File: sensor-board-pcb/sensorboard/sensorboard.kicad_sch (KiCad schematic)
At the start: 19 parts, among them J1 TO_MOTHERBOARD, J10 PZT_08, J11 PZT_09, J12 PZT_10, J13 PZT_11, J14 PZT_12, J15 PZT_13, J16 PZT_14, J17 PZT_15, J2 PZT_00, J3 PZT_01, J4 PZT_02, J5 PZT_03, J6 PZT_04, J7 PZT_05, J8 PZT_06, J9 PZT_07, U1 CD74HC4067M

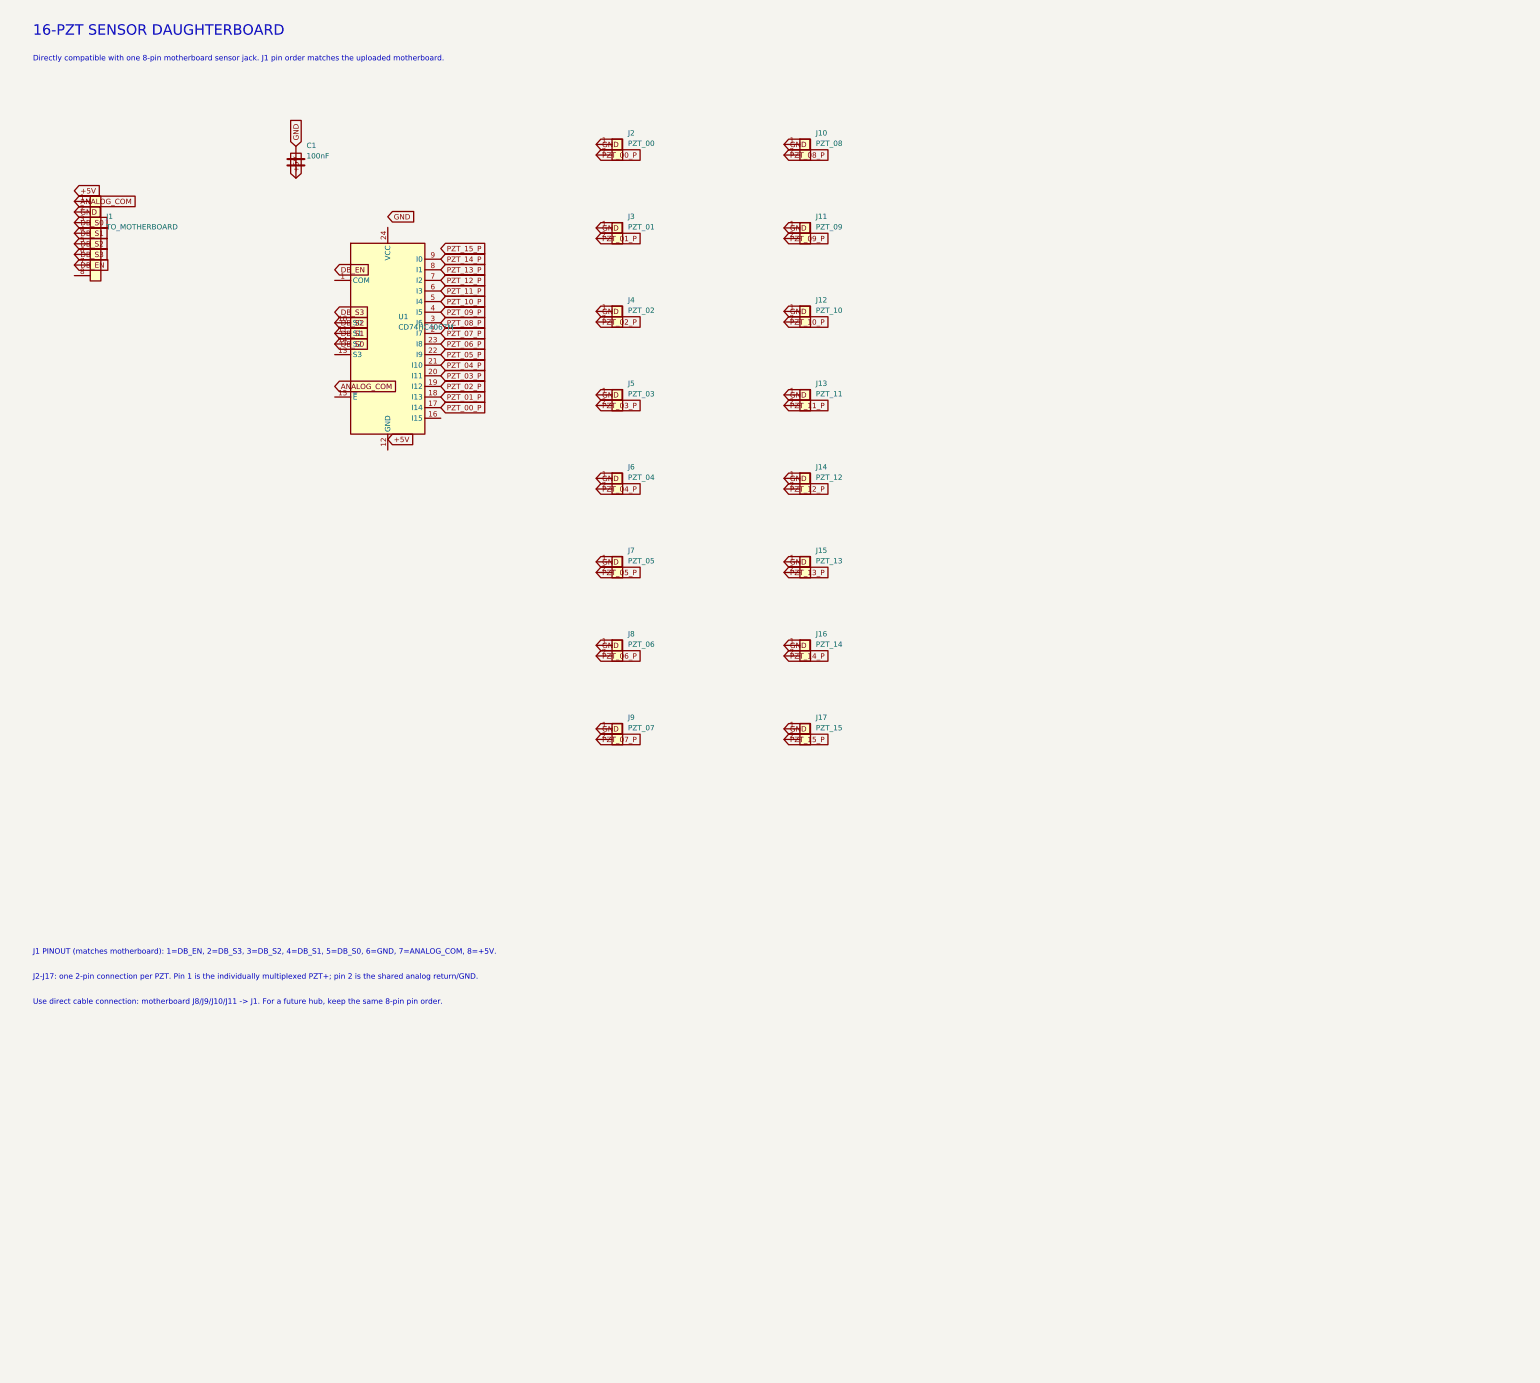
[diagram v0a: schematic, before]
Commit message: routing fixed
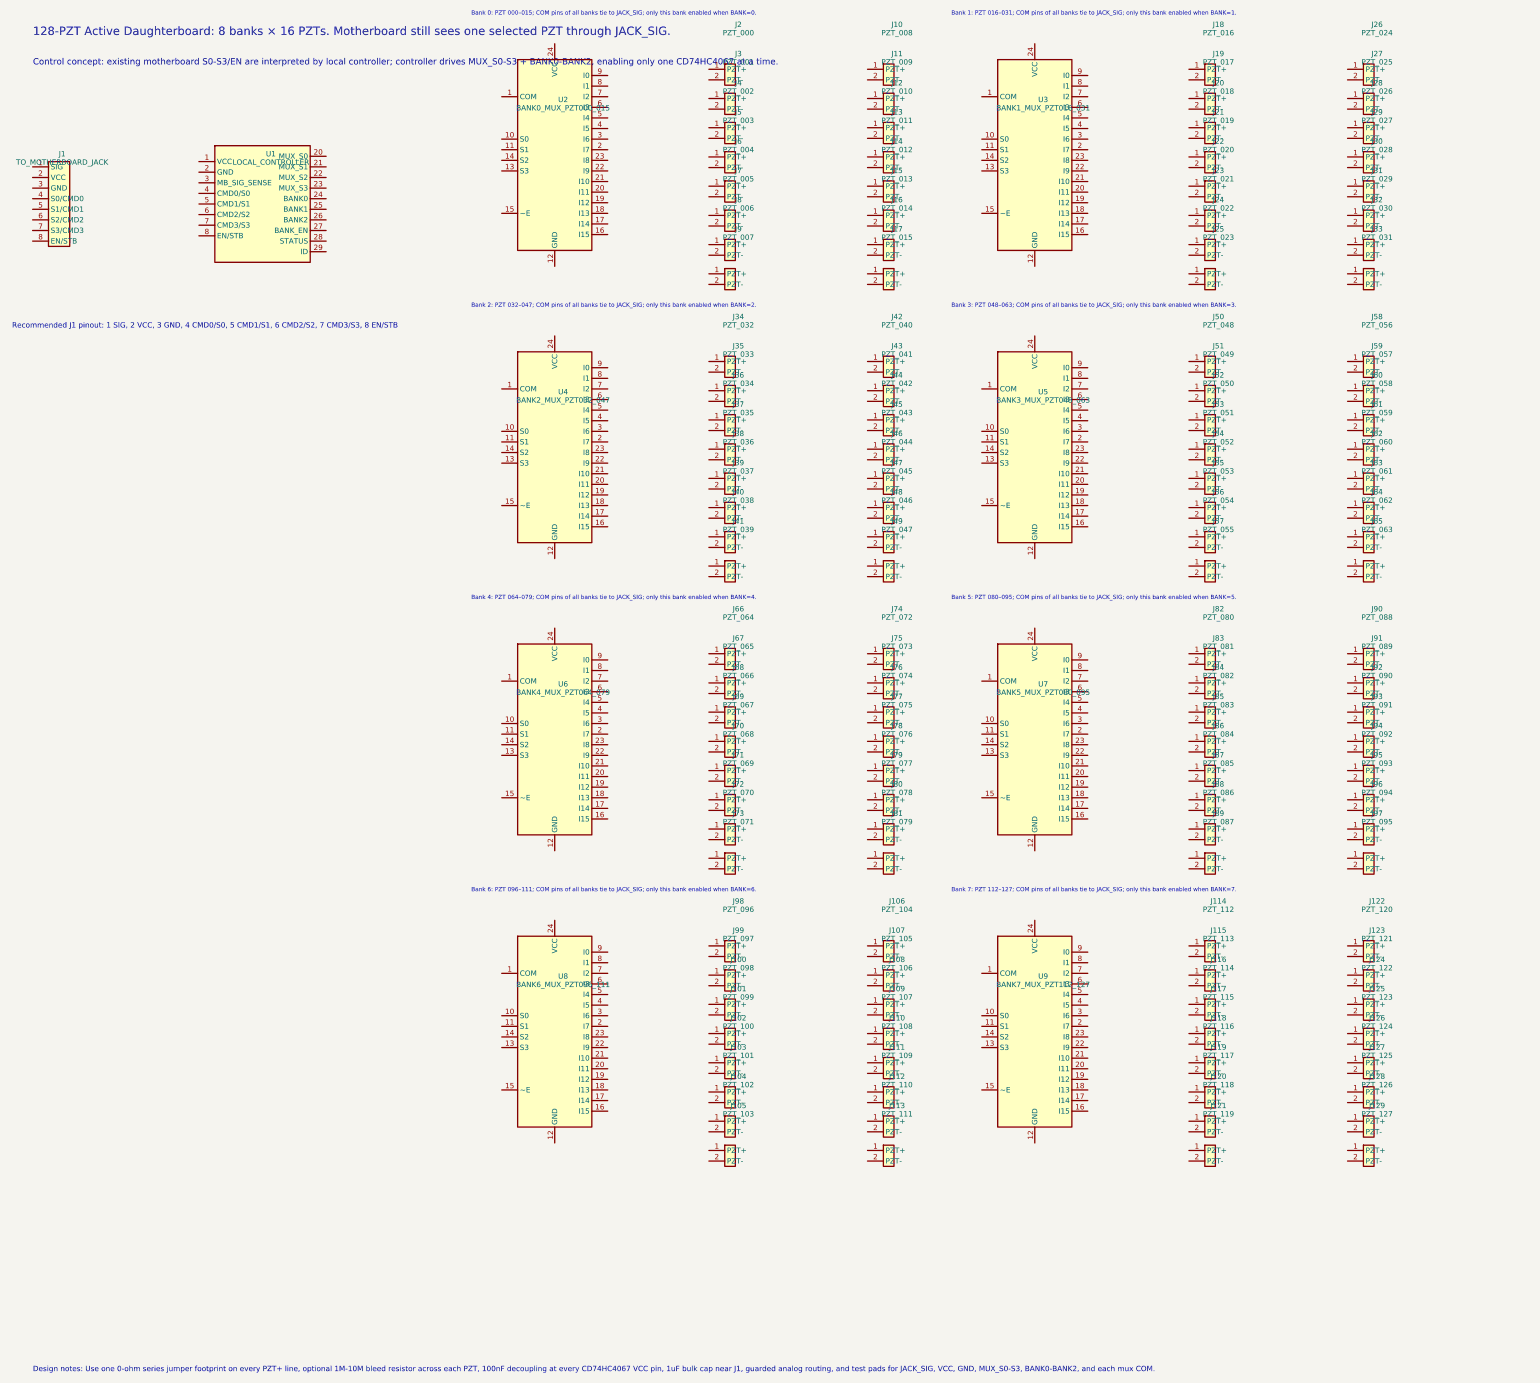
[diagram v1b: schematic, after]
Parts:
- removed C1: 100nF, Capacitor_SMD:C_0603_1608Metric, symbol Device:C
- removed J1: TO_MOTHERBOARD, Connector_Molex:Molex_Micro-Fit_3.0_43650-0815_1x08_P3.00mm_Vertical, symbol Connector_Generic:Conn_01x08
- removed J10: PZT_08, Connector_PinHeader_2.54mm:PinHeader_1x02_P2.54mm_Vertical, symbol Connector_Generic:Conn_01x02
- removed J11: PZT_09, Connector_PinHeader_2.54mm:PinHeader_1x02_P2.54mm_Vertical, symbol Connector_Generic:Conn_01x02
- removed J12: PZT_10, Connector_PinHeader_2.54mm:PinHeader_1x02_P2.54mm_Vertical, symbol Connector_Generic:Conn_01x02
- removed J13: PZT_11, Connector_PinHeader_2.54mm:PinHeader_1x02_P2.54mm_Vertical, symbol Connector_Generic:Conn_01x02
- removed J14: PZT_12, Connector_PinHeader_2.54mm:PinHeader_1x02_P2.54mm_Vertical, symbol Connector_Generic:Conn_01x02
- removed J15: PZT_13, Connector_PinHeader_2.54mm:PinHeader_1x02_P2.54mm_Vertical, symbol Connector_Generic:Conn_01x02
- removed J16: PZT_14, Connector_PinHeader_2.54mm:PinHeader_1x02_P2.54mm_Vertical, symbol Connector_Generic:Conn_01x02
- removed J17: PZT_15, Connector_PinHeader_2.54mm:PinHeader_1x02_P2.54mm_Vertical, symbol Connector_Generic:Conn_01x02
- removed J2: PZT_00, Connector_PinHeader_2.54mm:PinHeader_1x02_P2.54mm_Vertical, symbol Connector_Generic:Conn_01x02
- removed J3: PZT_01, Connector_PinHeader_2.54mm:PinHeader_1x02_P2.54mm_Vertical, symbol Connector_Generic:Conn_01x02
- removed J4: PZT_02, Connector_PinHeader_2.54mm:PinHeader_1x02_P2.54mm_Vertical, symbol Connector_Generic:Conn_01x02
- removed J5: PZT_03, Connector_PinHeader_2.54mm:PinHeader_1x02_P2.54mm_Vertical, symbol Connector_Generic:Conn_01x02
- removed J6: PZT_04, Connector_PinHeader_2.54mm:PinHeader_1x02_P2.54mm_Vertical, symbol Connector_Generic:Conn_01x02
- removed J7: PZT_05, Connector_PinHeader_2.54mm:PinHeader_1x02_P2.54mm_Vertical, symbol Connector_Generic:Conn_01x02
- removed J8: PZT_06, Connector_PinHeader_2.54mm:PinHeader_1x02_P2.54mm_Vertical, symbol Connector_Generic:Conn_01x02
- removed J9: PZT_07, Connector_PinHeader_2.54mm:PinHeader_1x02_P2.54mm_Vertical, symbol Connector_Generic:Conn_01x02
- removed U1: CD74HC4067M, Package_SO:SOIC-24W_7.5x15.4mm_P1.27mm, symbol 74xx:CD74HC4067M
- added J1: TO_MOTHERBOARD_JACK, Connector_PinHeader_2.54mm:PinHeader_1x08_P2.54mm_Vertical, symbol Daughter:MicroFit_01x08_Motherboard
- added J10: PZT_008, Connector_PinHeader_2.54mm:PinHeader_1x02_P2.54mm_Vertical, symbol Daughter:PZT_Conn_01x02
- added J100: PZT_098, Connector_PinHeader_2.54mm:PinHeader_1x02_P2.54mm_Vertical, symbol Daughter:PZT_Conn_01x02
- added J101: PZT_099, Connector_PinHeader_2.54mm:PinHeader_1x02_P2.54mm_Vertical, symbol Daughter:PZT_Conn_01x02
- added J102: PZT_100, Connector_PinHeader_2.54mm:PinHeader_1x02_P2.54mm_Vertical, symbol Daughter:PZT_Conn_01x02
- added J103: PZT_101, Connector_PinHeader_2.54mm:PinHeader_1x02_P2.54mm_Vertical, symbol Daughter:PZT_Conn_01x02
- added J104: PZT_102, Connector_PinHeader_2.54mm:PinHeader_1x02_P2.54mm_Vertical, symbol Daughter:PZT_Conn_01x02
- added J105: PZT_103, Connector_PinHeader_2.54mm:PinHeader_1x02_P2.54mm_Vertical, symbol Daughter:PZT_Conn_01x02
- added J106: PZT_104, Connector_PinHeader_2.54mm:PinHeader_1x02_P2.54mm_Vertical, symbol Daughter:PZT_Conn_01x02
- added J107: PZT_105, Connector_PinHeader_2.54mm:PinHeader_1x02_P2.54mm_Vertical, symbol Daughter:PZT_Conn_01x02
- added J108: PZT_106, Connector_PinHeader_2.54mm:PinHeader_1x02_P2.54mm_Vertical, symbol Daughter:PZT_Conn_01x02
- added J109: PZT_107, Connector_PinHeader_2.54mm:PinHeader_1x02_P2.54mm_Vertical, symbol Daughter:PZT_Conn_01x02
- added J11: PZT_009, Connector_PinHeader_2.54mm:PinHeader_1x02_P2.54mm_Vertical, symbol Daughter:PZT_Conn_01x02
- added J110: PZT_108, Connector_PinHeader_2.54mm:PinHeader_1x02_P2.54mm_Vertical, symbol Daughter:PZT_Conn_01x02
- added J111: PZT_109, Connector_PinHeader_2.54mm:PinHeader_1x02_P2.54mm_Vertical, symbol Daughter:PZT_Conn_01x02
- added J112: PZT_110, Connector_PinHeader_2.54mm:PinHeader_1x02_P2.54mm_Vertical, symbol Daughter:PZT_Conn_01x02
- added J113: PZT_111, Connector_PinHeader_2.54mm:PinHeader_1x02_P2.54mm_Vertical, symbol Daughter:PZT_Conn_01x02
- added J114: PZT_112, Connector_PinHeader_2.54mm:PinHeader_1x02_P2.54mm_Vertical, symbol Daughter:PZT_Conn_01x02
- added J115: PZT_113, Connector_PinHeader_2.54mm:PinHeader_1x02_P2.54mm_Vertical, symbol Daughter:PZT_Conn_01x02
- added J116: PZT_114, Connector_PinHeader_2.54mm:PinHeader_1x02_P2.54mm_Vertical, symbol Daughter:PZT_Conn_01x02
- added J117: PZT_115, Connector_PinHeader_2.54mm:PinHeader_1x02_P2.54mm_Vertical, symbol Daughter:PZT_Conn_01x02
- added J118: PZT_116, Connector_PinHeader_2.54mm:PinHeader_1x02_P2.54mm_Vertical, symbol Daughter:PZT_Conn_01x02
- added J119: PZT_117, Connector_PinHeader_2.54mm:PinHeader_1x02_P2.54mm_Vertical, symbol Daughter:PZT_Conn_01x02
- added J12: PZT_010, Connector_PinHeader_2.54mm:PinHeader_1x02_P2.54mm_Vertical, symbol Daughter:PZT_Conn_01x02
- added J120: PZT_118, Connector_PinHeader_2.54mm:PinHeader_1x02_P2.54mm_Vertical, symbol Daughter:PZT_Conn_01x02
- added J121: PZT_119, Connector_PinHeader_2.54mm:PinHeader_1x02_P2.54mm_Vertical, symbol Daughter:PZT_Conn_01x02
- added J122: PZT_120, Connector_PinHeader_2.54mm:PinHeader_1x02_P2.54mm_Vertical, symbol Daughter:PZT_Conn_01x02
- added J123: PZT_121, Connector_PinHeader_2.54mm:PinHeader_1x02_P2.54mm_Vertical, symbol Daughter:PZT_Conn_01x02
- added J124: PZT_122, Connector_PinHeader_2.54mm:PinHeader_1x02_P2.54mm_Vertical, symbol Daughter:PZT_Conn_01x02
- added J125: PZT_123, Connector_PinHeader_2.54mm:PinHeader_1x02_P2.54mm_Vertical, symbol Daughter:PZT_Conn_01x02
- added J126: PZT_124, Connector_PinHeader_2.54mm:PinHeader_1x02_P2.54mm_Vertical, symbol Daughter:PZT_Conn_01x02
- added J127: PZT_125, Connector_PinHeader_2.54mm:PinHeader_1x02_P2.54mm_Vertical, symbol Daughter:PZT_Conn_01x02
- added J128: PZT_126, Connector_PinHeader_2.54mm:PinHeader_1x02_P2.54mm_Vertical, symbol Daughter:PZT_Conn_01x02
- added J129: PZT_127, Connector_PinHeader_2.54mm:PinHeader_1x02_P2.54mm_Vertical, symbol Daughter:PZT_Conn_01x02
- added J13: PZT_011, Connector_PinHeader_2.54mm:PinHeader_1x02_P2.54mm_Vertical, symbol Daughter:PZT_Conn_01x02
- added J14: PZT_012, Connector_PinHeader_2.54mm:PinHeader_1x02_P2.54mm_Vertical, symbol Daughter:PZT_Conn_01x02
- added J15: PZT_013, Connector_PinHeader_2.54mm:PinHeader_1x02_P2.54mm_Vertical, symbol Daughter:PZT_Conn_01x02
- added J16: PZT_014, Connector_PinHeader_2.54mm:PinHeader_1x02_P2.54mm_Vertical, symbol Daughter:PZT_Conn_01x02
- added J17: PZT_015, Connector_PinHeader_2.54mm:PinHeader_1x02_P2.54mm_Vertical, symbol Daughter:PZT_Conn_01x02
- added J18: PZT_016, Connector_PinHeader_2.54mm:PinHeader_1x02_P2.54mm_Vertical, symbol Daughter:PZT_Conn_01x02
- added J19: PZT_017, Connector_PinHeader_2.54mm:PinHeader_1x02_P2.54mm_Vertical, symbol Daughter:PZT_Conn_01x02
- added J2: PZT_000, Connector_PinHeader_2.54mm:PinHeader_1x02_P2.54mm_Vertical, symbol Daughter:PZT_Conn_01x02
- added J20: PZT_018, Connector_PinHeader_2.54mm:PinHeader_1x02_P2.54mm_Vertical, symbol Daughter:PZT_Conn_01x02
- added J21: PZT_019, Connector_PinHeader_2.54mm:PinHeader_1x02_P2.54mm_Vertical, symbol Daughter:PZT_Conn_01x02
- added J22: PZT_020, Connector_PinHeader_2.54mm:PinHeader_1x02_P2.54mm_Vertical, symbol Daughter:PZT_Conn_01x02
- added J23: PZT_021, Connector_PinHeader_2.54mm:PinHeader_1x02_P2.54mm_Vertical, symbol Daughter:PZT_Conn_01x02
- added J24: PZT_022, Connector_PinHeader_2.54mm:PinHeader_1x02_P2.54mm_Vertical, symbol Daughter:PZT_Conn_01x02
- added J25: PZT_023, Connector_PinHeader_2.54mm:PinHeader_1x02_P2.54mm_Vertical, symbol Daughter:PZT_Conn_01x02
- added J26: PZT_024, Connector_PinHeader_2.54mm:PinHeader_1x02_P2.54mm_Vertical, symbol Daughter:PZT_Conn_01x02
- added J27: PZT_025, Connector_PinHeader_2.54mm:PinHeader_1x02_P2.54mm_Vertical, symbol Daughter:PZT_Conn_01x02
- added J28: PZT_026, Connector_PinHeader_2.54mm:PinHeader_1x02_P2.54mm_Vertical, symbol Daughter:PZT_Conn_01x02
- added J29: PZT_027, Connector_PinHeader_2.54mm:PinHeader_1x02_P2.54mm_Vertical, symbol Daughter:PZT_Conn_01x02
- added J3: PZT_001, Connector_PinHeader_2.54mm:PinHeader_1x02_P2.54mm_Vertical, symbol Daughter:PZT_Conn_01x02
- added J30: PZT_028, Connector_PinHeader_2.54mm:PinHeader_1x02_P2.54mm_Vertical, symbol Daughter:PZT_Conn_01x02
- added J31: PZT_029, Connector_PinHeader_2.54mm:PinHeader_1x02_P2.54mm_Vertical, symbol Daughter:PZT_Conn_01x02
- added J32: PZT_030, Connector_PinHeader_2.54mm:PinHeader_1x02_P2.54mm_Vertical, symbol Daughter:PZT_Conn_01x02
- added J33: PZT_031, Connector_PinHeader_2.54mm:PinHeader_1x02_P2.54mm_Vertical, symbol Daughter:PZT_Conn_01x02
- added J34: PZT_032, Connector_PinHeader_2.54mm:PinHeader_1x02_P2.54mm_Vertical, symbol Daughter:PZT_Conn_01x02
- added J35: PZT_033, Connector_PinHeader_2.54mm:PinHeader_1x02_P2.54mm_Vertical, symbol Daughter:PZT_Conn_01x02
- added J36: PZT_034, Connector_PinHeader_2.54mm:PinHeader_1x02_P2.54mm_Vertical, symbol Daughter:PZT_Conn_01x02
- added J37: PZT_035, Connector_PinHeader_2.54mm:PinHeader_1x02_P2.54mm_Vertical, symbol Daughter:PZT_Conn_01x02
- added J38: PZT_036, Connector_PinHeader_2.54mm:PinHeader_1x02_P2.54mm_Vertical, symbol Daughter:PZT_Conn_01x02
- added J39: PZT_037, Connector_PinHeader_2.54mm:PinHeader_1x02_P2.54mm_Vertical, symbol Daughter:PZT_Conn_01x02
- added J4: PZT_002, Connector_PinHeader_2.54mm:PinHeader_1x02_P2.54mm_Vertical, symbol Daughter:PZT_Conn_01x02
- added J40: PZT_038, Connector_PinHeader_2.54mm:PinHeader_1x02_P2.54mm_Vertical, symbol Daughter:PZT_Conn_01x02
- added J41: PZT_039, Connector_PinHeader_2.54mm:PinHeader_1x02_P2.54mm_Vertical, symbol Daughter:PZT_Conn_01x02
- added J42: PZT_040, Connector_PinHeader_2.54mm:PinHeader_1x02_P2.54mm_Vertical, symbol Daughter:PZT_Conn_01x02
- added J43: PZT_041, Connector_PinHeader_2.54mm:PinHeader_1x02_P2.54mm_Vertical, symbol Daughter:PZT_Conn_01x02
- added J44: PZT_042, Connector_PinHeader_2.54mm:PinHeader_1x02_P2.54mm_Vertical, symbol Daughter:PZT_Conn_01x02
- added J45: PZT_043, Connector_PinHeader_2.54mm:PinHeader_1x02_P2.54mm_Vertical, symbol Daughter:PZT_Conn_01x02
- added J46: PZT_044, Connector_PinHeader_2.54mm:PinHeader_1x02_P2.54mm_Vertical, symbol Daughter:PZT_Conn_01x02
- added J47: PZT_045, Connector_PinHeader_2.54mm:PinHeader_1x02_P2.54mm_Vertical, symbol Daughter:PZT_Conn_01x02
- added J48: PZT_046, Connector_PinHeader_2.54mm:PinHeader_1x02_P2.54mm_Vertical, symbol Daughter:PZT_Conn_01x02
- added J49: PZT_047, Connector_PinHeader_2.54mm:PinHeader_1x02_P2.54mm_Vertical, symbol Daughter:PZT_Conn_01x02
- added J5: PZT_003, Connector_PinHeader_2.54mm:PinHeader_1x02_P2.54mm_Vertical, symbol Daughter:PZT_Conn_01x02
- added J50: PZT_048, Connector_PinHeader_2.54mm:PinHeader_1x02_P2.54mm_Vertical, symbol Daughter:PZT_Conn_01x02
- added J51: PZT_049, Connector_PinHeader_2.54mm:PinHeader_1x02_P2.54mm_Vertical, symbol Daughter:PZT_Conn_01x02
- added J52: PZT_050, Connector_PinHeader_2.54mm:PinHeader_1x02_P2.54mm_Vertical, symbol Daughter:PZT_Conn_01x02
- added J53: PZT_051, Connector_PinHeader_2.54mm:PinHeader_1x02_P2.54mm_Vertical, symbol Daughter:PZT_Conn_01x02
- added J54: PZT_052, Connector_PinHeader_2.54mm:PinHeader_1x02_P2.54mm_Vertical, symbol Daughter:PZT_Conn_01x02
- added J55: PZT_053, Connector_PinHeader_2.54mm:PinHeader_1x02_P2.54mm_Vertical, symbol Daughter:PZT_Conn_01x02
- added J56: PZT_054, Connector_PinHeader_2.54mm:PinHeader_1x02_P2.54mm_Vertical, symbol Daughter:PZT_Conn_01x02
- added J57: PZT_055, Connector_PinHeader_2.54mm:PinHeader_1x02_P2.54mm_Vertical, symbol Daughter:PZT_Conn_01x02
- added J58: PZT_056, Connector_PinHeader_2.54mm:PinHeader_1x02_P2.54mm_Vertical, symbol Daughter:PZT_Conn_01x02
- added J59: PZT_057, Connector_PinHeader_2.54mm:PinHeader_1x02_P2.54mm_Vertical, symbol Daughter:PZT_Conn_01x02
- added J6: PZT_004, Connector_PinHeader_2.54mm:PinHeader_1x02_P2.54mm_Vertical, symbol Daughter:PZT_Conn_01x02
- added J60: PZT_058, Connector_PinHeader_2.54mm:PinHeader_1x02_P2.54mm_Vertical, symbol Daughter:PZT_Conn_01x02
- added J61: PZT_059, Connector_PinHeader_2.54mm:PinHeader_1x02_P2.54mm_Vertical, symbol Daughter:PZT_Conn_01x02
- added J62: PZT_060, Connector_PinHeader_2.54mm:PinHeader_1x02_P2.54mm_Vertical, symbol Daughter:PZT_Conn_01x02
- added J63: PZT_061, Connector_PinHeader_2.54mm:PinHeader_1x02_P2.54mm_Vertical, symbol Daughter:PZT_Conn_01x02
- added J64: PZT_062, Connector_PinHeader_2.54mm:PinHeader_1x02_P2.54mm_Vertical, symbol Daughter:PZT_Conn_01x02
- added J65: PZT_063, Connector_PinHeader_2.54mm:PinHeader_1x02_P2.54mm_Vertical, symbol Daughter:PZT_Conn_01x02
- added J66: PZT_064, Connector_PinHeader_2.54mm:PinHeader_1x02_P2.54mm_Vertical, symbol Daughter:PZT_Conn_01x02
- added J67: PZT_065, Connector_PinHeader_2.54mm:PinHeader_1x02_P2.54mm_Vertical, symbol Daughter:PZT_Conn_01x02
- added J68: PZT_066, Connector_PinHeader_2.54mm:PinHeader_1x02_P2.54mm_Vertical, symbol Daughter:PZT_Conn_01x02
- added J69: PZT_067, Connector_PinHeader_2.54mm:PinHeader_1x02_P2.54mm_Vertical, symbol Daughter:PZT_Conn_01x02
- added J7: PZT_005, Connector_PinHeader_2.54mm:PinHeader_1x02_P2.54mm_Vertical, symbol Daughter:PZT_Conn_01x02
- added J70: PZT_068, Connector_PinHeader_2.54mm:PinHeader_1x02_P2.54mm_Vertical, symbol Daughter:PZT_Conn_01x02
- added J71: PZT_069, Connector_PinHeader_2.54mm:PinHeader_1x02_P2.54mm_Vertical, symbol Daughter:PZT_Conn_01x02
- added J72: PZT_070, Connector_PinHeader_2.54mm:PinHeader_1x02_P2.54mm_Vertical, symbol Daughter:PZT_Conn_01x02
- added J73: PZT_071, Connector_PinHeader_2.54mm:PinHeader_1x02_P2.54mm_Vertical, symbol Daughter:PZT_Conn_01x02
- added J74: PZT_072, Connector_PinHeader_2.54mm:PinHeader_1x02_P2.54mm_Vertical, symbol Daughter:PZT_Conn_01x02
- added J75: PZT_073, Connector_PinHeader_2.54mm:PinHeader_1x02_P2.54mm_Vertical, symbol Daughter:PZT_Conn_01x02
- added J76: PZT_074, Connector_PinHeader_2.54mm:PinHeader_1x02_P2.54mm_Vertical, symbol Daughter:PZT_Conn_01x02
- added J77: PZT_075, Connector_PinHeader_2.54mm:PinHeader_1x02_P2.54mm_Vertical, symbol Daughter:PZT_Conn_01x02
- added J78: PZT_076, Connector_PinHeader_2.54mm:PinHeader_1x02_P2.54mm_Vertical, symbol Daughter:PZT_Conn_01x02
- added J79: PZT_077, Connector_PinHeader_2.54mm:PinHeader_1x02_P2.54mm_Vertical, symbol Daughter:PZT_Conn_01x02
- added J8: PZT_006, Connector_PinHeader_2.54mm:PinHeader_1x02_P2.54mm_Vertical, symbol Daughter:PZT_Conn_01x02
- added J80: PZT_078, Connector_PinHeader_2.54mm:PinHeader_1x02_P2.54mm_Vertical, symbol Daughter:PZT_Conn_01x02
- added J81: PZT_079, Connector_PinHeader_2.54mm:PinHeader_1x02_P2.54mm_Vertical, symbol Daughter:PZT_Conn_01x02
- added J82: PZT_080, Connector_PinHeader_2.54mm:PinHeader_1x02_P2.54mm_Vertical, symbol Daughter:PZT_Conn_01x02
- added J83: PZT_081, Connector_PinHeader_2.54mm:PinHeader_1x02_P2.54mm_Vertical, symbol Daughter:PZT_Conn_01x02
- added J84: PZT_082, Connector_PinHeader_2.54mm:PinHeader_1x02_P2.54mm_Vertical, symbol Daughter:PZT_Conn_01x02
- added J85: PZT_083, Connector_PinHeader_2.54mm:PinHeader_1x02_P2.54mm_Vertical, symbol Daughter:PZT_Conn_01x02
- added J86: PZT_084, Connector_PinHeader_2.54mm:PinHeader_1x02_P2.54mm_Vertical, symbol Daughter:PZT_Conn_01x02
- added J87: PZT_085, Connector_PinHeader_2.54mm:PinHeader_1x02_P2.54mm_Vertical, symbol Daughter:PZT_Conn_01x02
- added J88: PZT_086, Connector_PinHeader_2.54mm:PinHeader_1x02_P2.54mm_Vertical, symbol Daughter:PZT_Conn_01x02
- added J89: PZT_087, Connector_PinHeader_2.54mm:PinHeader_1x02_P2.54mm_Vertical, symbol Daughter:PZT_Conn_01x02
- added J9: PZT_007, Connector_PinHeader_2.54mm:PinHeader_1x02_P2.54mm_Vertical, symbol Daughter:PZT_Conn_01x02
- added J90: PZT_088, Connector_PinHeader_2.54mm:PinHeader_1x02_P2.54mm_Vertical, symbol Daughter:PZT_Conn_01x02
- added J91: PZT_089, Connector_PinHeader_2.54mm:PinHeader_1x02_P2.54mm_Vertical, symbol Daughter:PZT_Conn_01x02
- added J92: PZT_090, Connector_PinHeader_2.54mm:PinHeader_1x02_P2.54mm_Vertical, symbol Daughter:PZT_Conn_01x02
- added J93: PZT_091, Connector_PinHeader_2.54mm:PinHeader_1x02_P2.54mm_Vertical, symbol Daughter:PZT_Conn_01x02
- added J94: PZT_092, Connector_PinHeader_2.54mm:PinHeader_1x02_P2.54mm_Vertical, symbol Daughter:PZT_Conn_01x02
- added J95: PZT_093, Connector_PinHeader_2.54mm:PinHeader_1x02_P2.54mm_Vertical, symbol Daughter:PZT_Conn_01x02
- added J96: PZT_094, Connector_PinHeader_2.54mm:PinHeader_1x02_P2.54mm_Vertical, symbol Daughter:PZT_Conn_01x02
- added J97: PZT_095, Connector_PinHeader_2.54mm:PinHeader_1x02_P2.54mm_Vertical, symbol Daughter:PZT_Conn_01x02
- added J98: PZT_096, Connector_PinHeader_2.54mm:PinHeader_1x02_P2.54mm_Vertical, symbol Daughter:PZT_Conn_01x02
- added J99: PZT_097, Connector_PinHeader_2.54mm:PinHeader_1x02_P2.54mm_Vertical, symbol Daughter:PZT_Conn_01x02
- added U1: LOCAL_CONTROLLER, Package_DIP:DIP-20_W7.62mm, symbol Daughter:Local_Controller_or_GPIO
- added U2: BANK0_MUX_PZT000_015, Package_SO:SOIC-24W_7.5x15.4mm_P1.27mm, symbol Daughter:CD74HC4067M
- added U3: BANK1_MUX_PZT016_031, Package_SO:SOIC-24W_7.5x15.4mm_P1.27mm, symbol Daughter:CD74HC4067M
- added U4: BANK2_MUX_PZT032_047, Package_SO:SOIC-24W_7.5x15.4mm_P1.27mm, symbol Daughter:CD74HC4067M
- added U5: BANK3_MUX_PZT048_063, Package_SO:SOIC-24W_7.5x15.4mm_P1.27mm, symbol Daughter:CD74HC4067M
- added U6: BANK4_MUX_PZT064_079, Package_SO:SOIC-24W_7.5x15.4mm_P1.27mm, symbol Daughter:CD74HC4067M
- added U7: BANK5_MUX_PZT080_095, Package_SO:SOIC-24W_7.5x15.4mm_P1.27mm, symbol Daughter:CD74HC4067M
- added U8: BANK6_MUX_PZT096_111, Package_SO:SOIC-24W_7.5x15.4mm_P1.27mm, symbol Daughter:CD74HC4067M
- added U9: BANK7_MUX_PZT112_127, Package_SO:SOIC-24W_7.5x15.4mm_P1.27mm, symbol Daughter:CD74HC4067M
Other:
- note added: "128-PZT Active Daughterboard: 8 banks × 16 PZTs. Motherboard still sees one selected PZT through JACK_SIG."
- note added: "Bank 0: PZT 000–015; COM pins of all banks tie to JACK_SIG; only this bank enabled when BANK=0."
- note added: "Bank 1: PZT 016–031; COM pins of all banks tie to JACK_SIG; only this bank enabled when BANK=1."
- note added: "Bank 2: PZT 032–047; COM pins of all banks tie to JACK_SIG; only this bank enabled when BANK=2."
- note added: "Bank 3: PZT 048–063; COM pins of all banks tie to JACK_SIG; only this bank enabled when BANK=3."
- note added: "Bank 4: PZT 064–079; COM pins of all banks tie to JACK_SIG; only this bank enabled when BANK=4."
- note added: "Bank 5: PZT 080–095; COM pins of all banks tie to JACK_SIG; only this bank enabled when BANK=5."
- note added: "Bank 6: PZT 096–111; COM pins of all banks tie to JACK_SIG; only this bank enabled when BANK=6."
- note added: "Bank 7: PZT 112–127; COM pins of all banks tie to JACK_SIG; only this bank enabled when BANK=7."
- note added: "Control concept: existing motherboard S0-S3/EN are interpreted by local controller; controller drives MUX_S0-S3 + BANK0-BANK2, enabling only one CD74HC4067 at a time."
- note added: "Design notes: Use one 0-ohm series jumper footprint on every PZT+ line, optional 1M-10M bleed resistor across each PZT, 100nF decoupling at every CD74HC4067 VCC pin, 1uF bulk cap near J1, guarded analog routing, and test pads for JACK_SIG, VCC, GND, MUX_S0-S3, BANK0-BANK2, and each mux COM."
- note added: "Recommended J1 pinout: 1 SIG, 2 VCC, 3 GND, 4 CMD0/S0, 5 CMD1/S1, 6 CMD2/S2, 7 CMD3/S3, 8 EN/STB"
- note removed: "16-PZT SENSOR DAUGHTERBOARD"
- note removed: "Directly compatible with one 8-pin motherboard sensor jack. J1 pin order matches the uploaded motherboard."
- note removed: "J1 PINOUT (matches motherboard): 1=DB_EN, 2=DB_S3, 3=DB_S2, 4=DB_S1, 5=DB_S0, 6=GND, 7=ANALOG_COM, 8=+5V."
- note removed: "J2-J17: one 2-pin connection per PZT. Pin 1 is the individually multiplexed PZT+; pin 2 is the shared analog return/GND."
- note removed: "Use direct cable connection: motherboard J8/J9/J10/J11 -> J1. For a future hub, keep the same 8-pin pin order."
